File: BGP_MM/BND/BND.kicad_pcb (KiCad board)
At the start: 2 copper layers, 27 x 28 mm, 5 parts, among them J1 Conn_01x02, J2 Conn_01x03, P1 CONN_01X04, P2 Conn_01x02

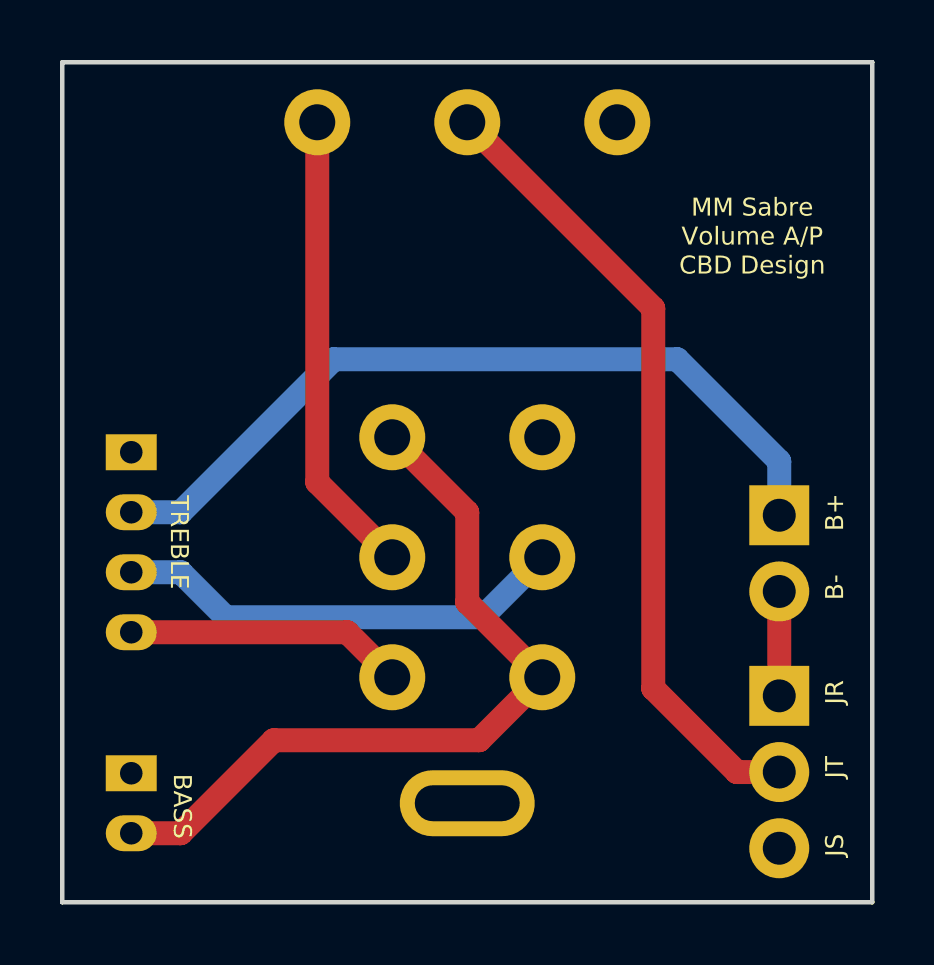
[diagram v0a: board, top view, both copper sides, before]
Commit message: MM Refactoring
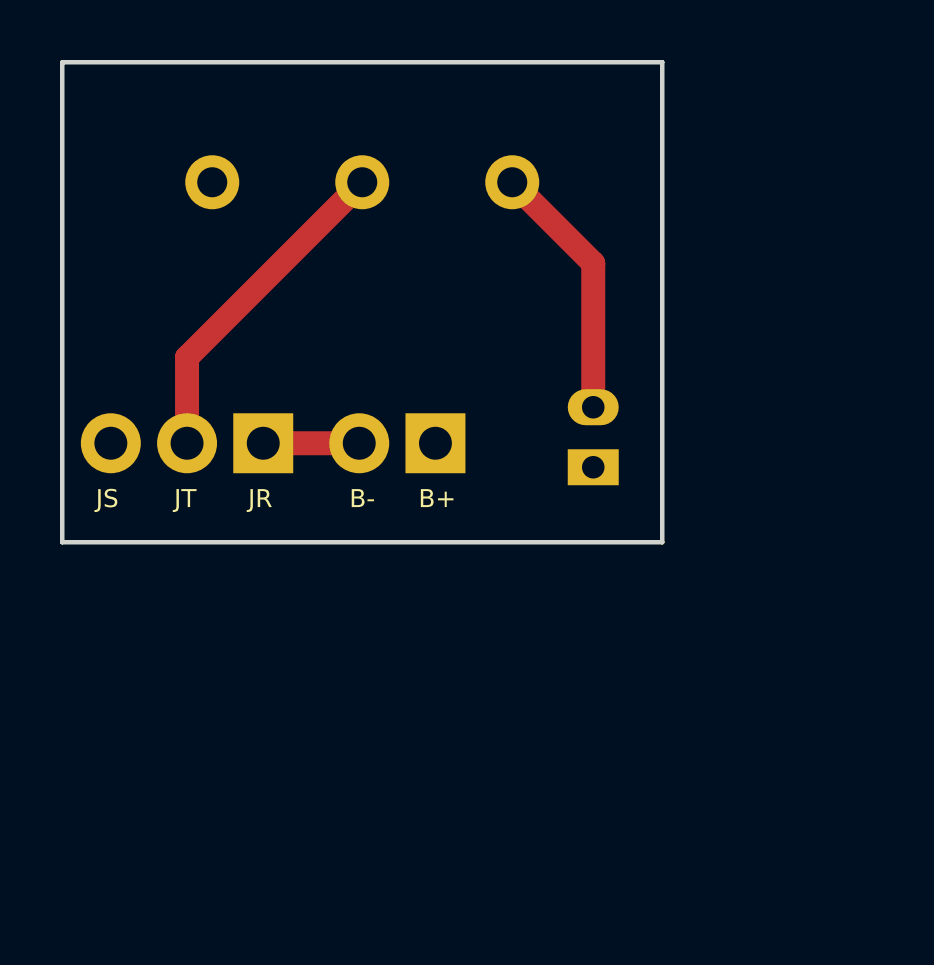
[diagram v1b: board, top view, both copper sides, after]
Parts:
- removed P2: Conn_01x02, Connectors_JST:JST_PH_B2B-PH-K_02x2.00mm_Straight
- P1: value CONN_01X04 -> CONN_01X02; footprint Connectors_JST:JST_PH_B4B-PH-K_04x2.00mm_Straight -> Connectors_JST:JST_PH_B2B-PH-K_02x2.00mm_Straight
- RV1: value CONN_01X10 -> POT; footprint LIBS:Bournes_Blend_PP_PCB -> LIBS:Potentiometer_Alpha_RV16
- moved J2 19.2 mm to (109.7, 82.7), turned to 180 degrees
- moved P1 15.4 mm to (120.7, 83.5), turned to 90 degrees
- moved J1 11.7 mm to (115.4, 82.7), turned to 180 degrees
- moved RV1 2.50 mm to (113.0, 74.0)
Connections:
- P1 pad 2: VCC -> Net-(P1-Pad2)
- RV1 pad 1: /VOL_I -> Earth
- RV1 pad 3: Earth -> Net-(P1-Pad2)
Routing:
- net VCC: track 26.9 -> 0.00 mm
- net /PSV_I: track 25.9 -> 0.00 mm
- net /OUT: track 26.8 -> 11.1 mm
- net /VOL_I: track 15.5 -> 0.00 mm
- net /ACT_O: track 15.1 -> 0.00 mm
- net /ACT_I: track 9.32 -> 0.00 mm
- net Net-(P1-Pad2): track 0.00 -> 8.62 mm
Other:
- board size 27 x 28 mm -> 20 x 16 mm
- board text removed: "BASS"
- board text removed: "MM Sabre Volume A/P CBD Design"
- board text removed: "TREBLE"

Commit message: MM Refactoring
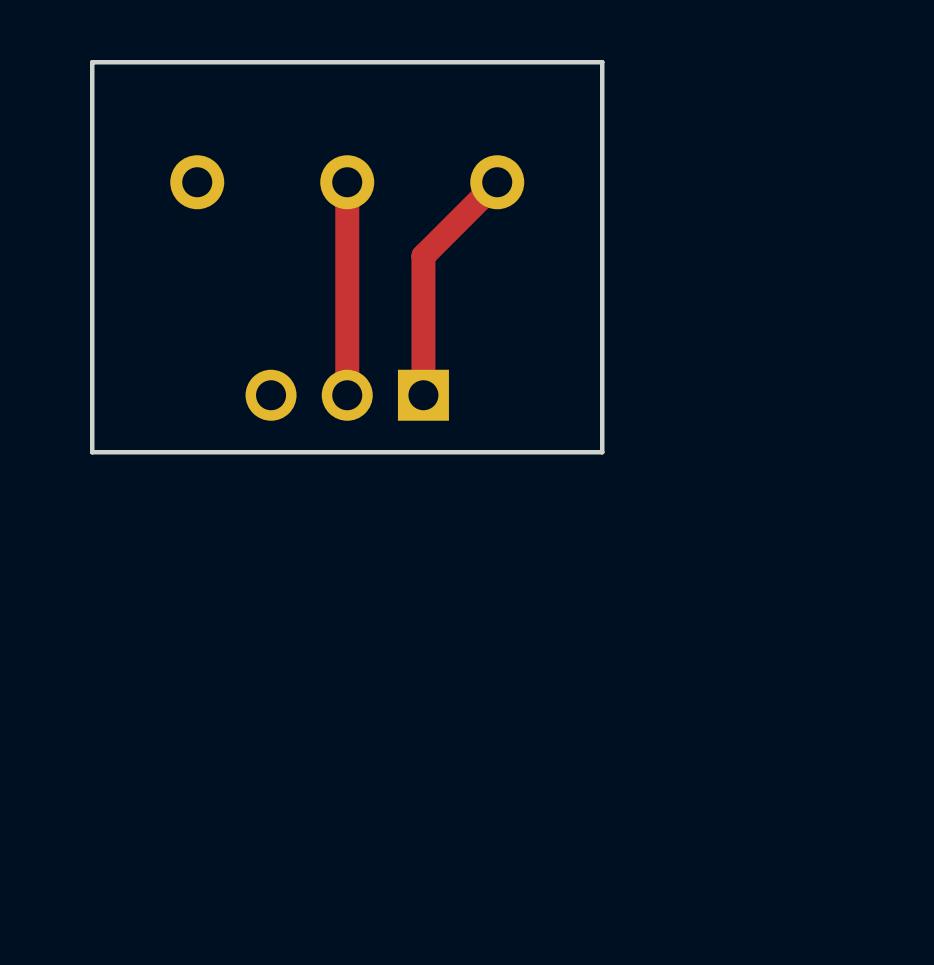
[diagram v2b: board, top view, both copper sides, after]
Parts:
- removed J2: Conn_01x03, Terminal_Blocks:TerminalBlock_Pheonix_MPT-2.54mm_3pol
- removed P1: CONN_01X02, Connectors_JST:JST_PH_B2B-PH-K_02x2.00mm_Straight
- J1: value Conn_01x02 -> Conn_01x03_Male; footprint Terminal_Blocks:TerminalBlock_Pheonix_MPT-2.54mm_2pol -> Pin_Headers:Pin_Header_Straight_1x03_Pitch2.54mm
- moved J1 1.65 mm to (115.0, 81.1), turned to 90 degrees
- moved RV1 0.50 mm to (112.5, 74.0)
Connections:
- J1 pad 1: VCC -> /IN
- J1 pad 2: Net-(J1-Pad2) -> /OUT
- RV1 pad 3: Net-(P1-Pad2) -> /IN
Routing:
- net Net-(P1-Pad2): track 8.62 -> 0.00 mm
- net /IN: track 0.00 -> 8.02 mm
- net /OUT: track 11.1 -> 7.00 mm
- net Net-(J1-Pad2): track 3.20 -> 0.00 mm
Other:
- board size 20 x 16 mm -> 17 x 13 mm
- board text removed: "B+"
- board text removed: "B-"
- board text removed: "JR"
- board text removed: "JS"
- board text removed: "JT"
